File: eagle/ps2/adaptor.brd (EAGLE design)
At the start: 100 x 80 mm, 9 parts, among them T1 BSS138, T3 BSS138

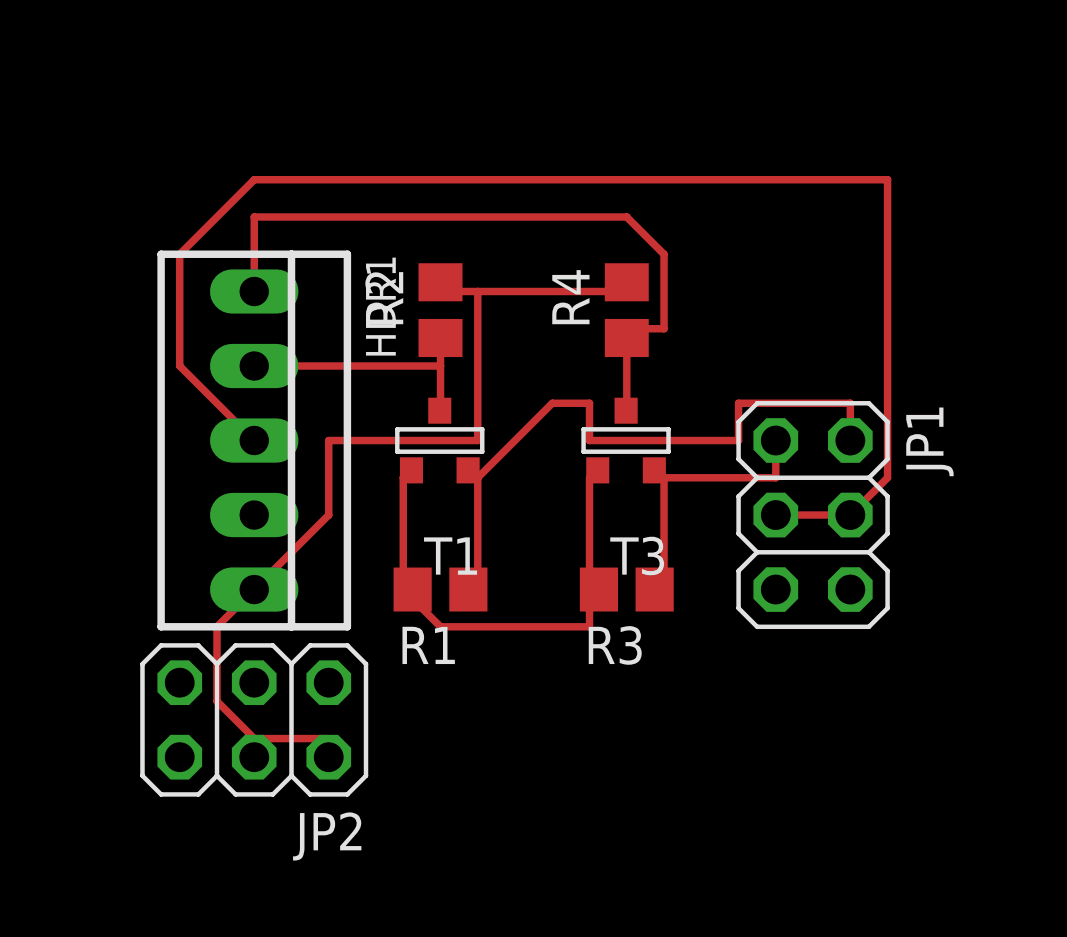
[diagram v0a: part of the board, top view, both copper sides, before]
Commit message: updated
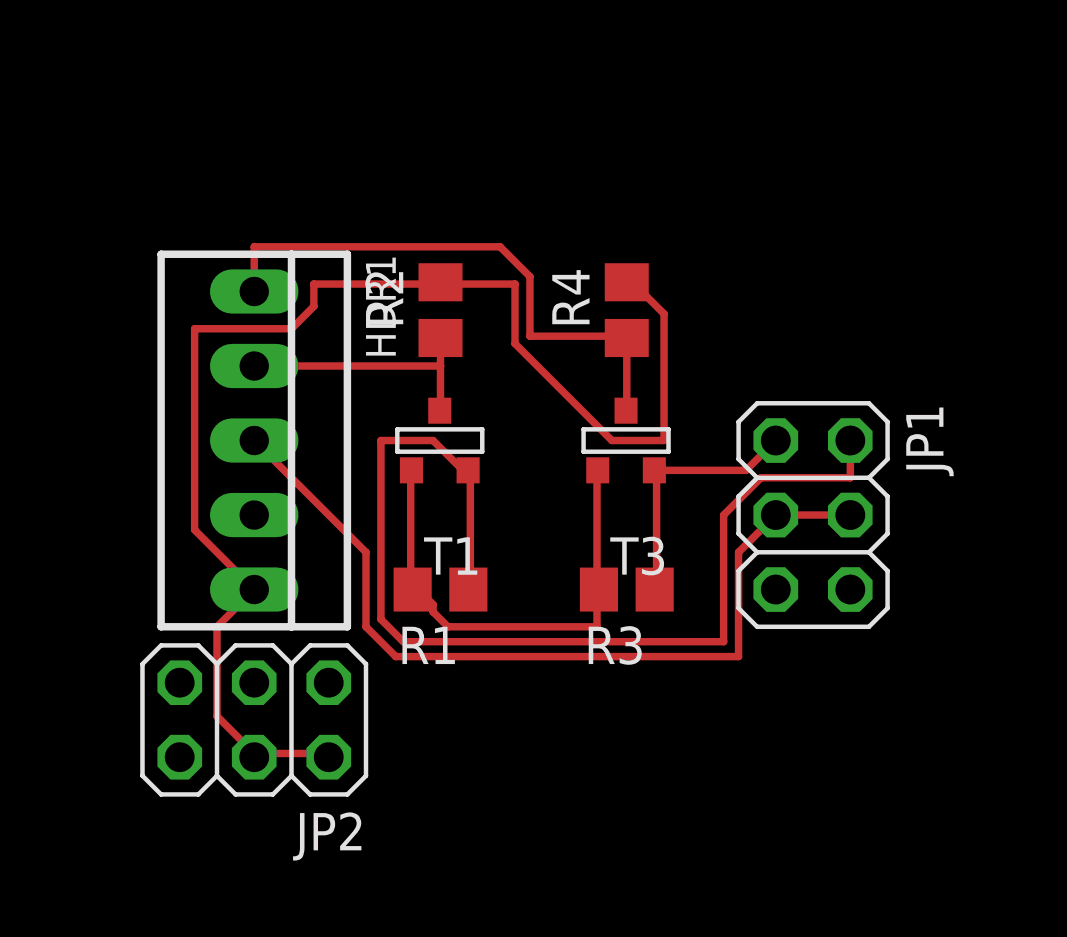
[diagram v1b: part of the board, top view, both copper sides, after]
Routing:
- net GND: track 47.1 -> 28.9 mm
- net CLK_3V3: track 22.1 -> 36.1 mm
- net VCC_5V: track 33.2 -> 46.0 mm
- net DATA_5V: track 23.6 -> 19.2 mm
- net DATA_3V3: track 9.63 -> 8.69 mm
- net VCC_3V3: track 17.2 -> 16.5 mm
